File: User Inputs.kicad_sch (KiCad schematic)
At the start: 10 parts, among them SW3 RotaryEncoder_Switch

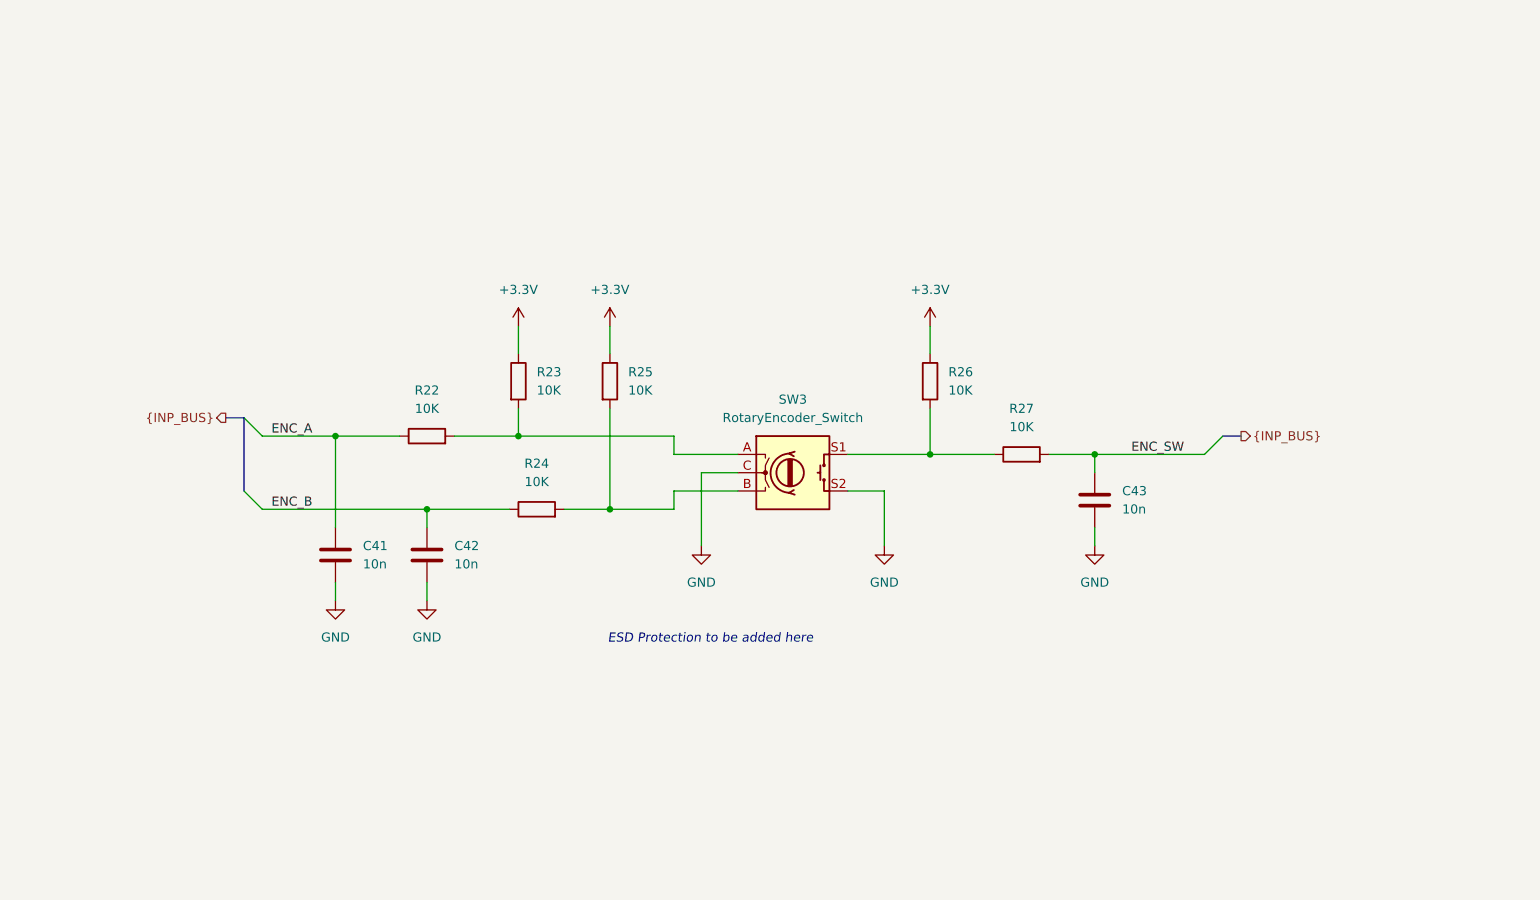
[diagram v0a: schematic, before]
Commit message: Major Changes
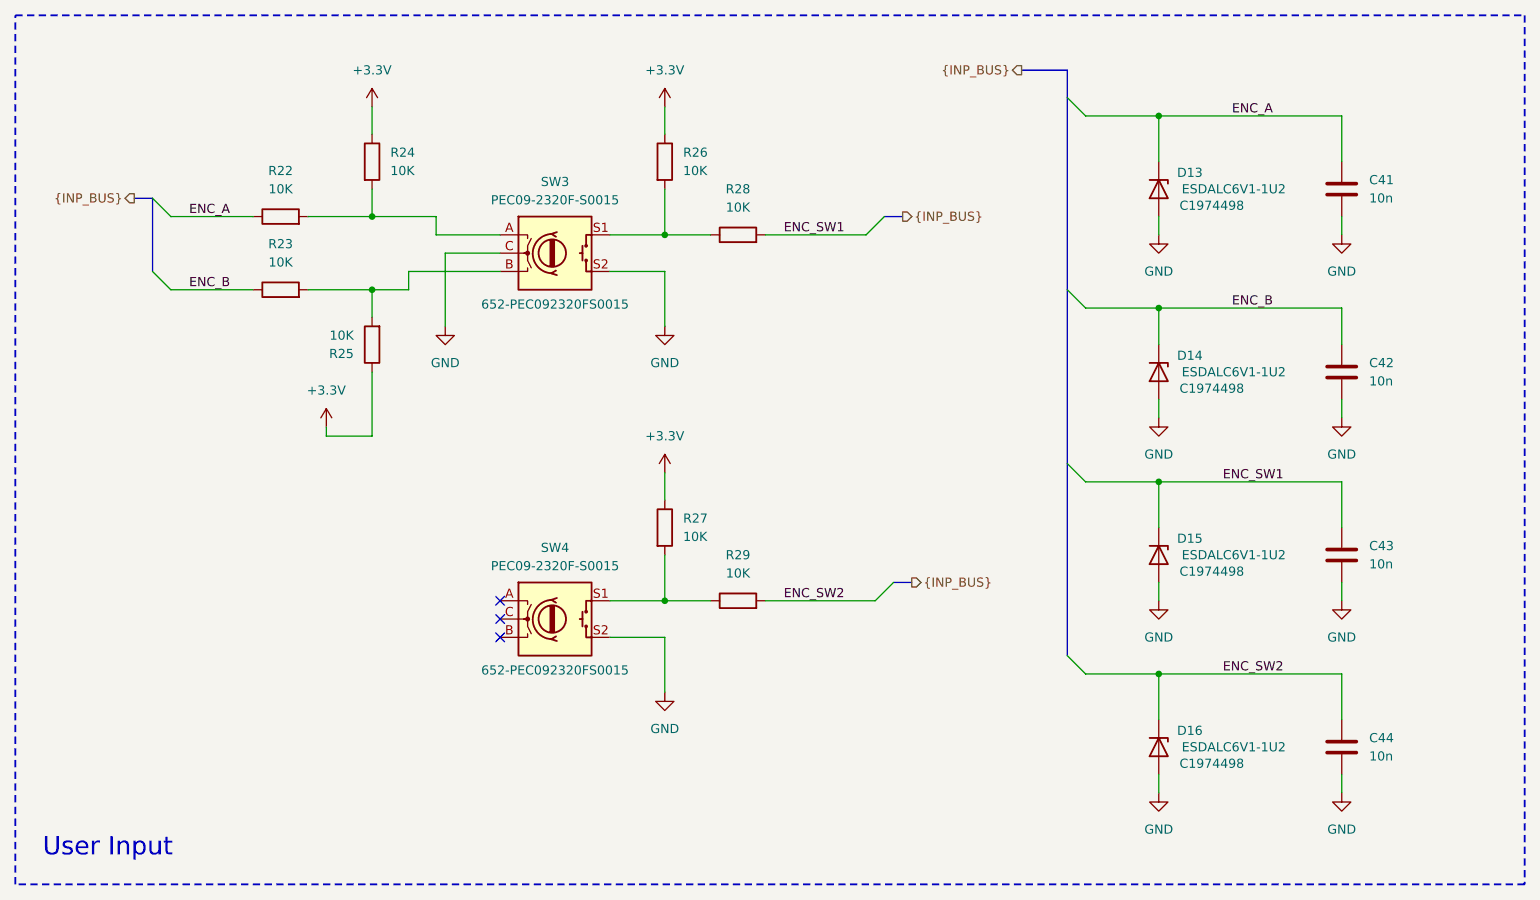
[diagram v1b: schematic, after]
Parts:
- added C44: 10n, Capacitor_SMD:C_0402_1005Metric, symbol Device:C
- added D13, D14, D15, D16: ESDALC6V1-1U2, precision_clock:ST ESDALC6V1-1U2, symbol Diode:ESD5Zxx
- added R27, R29: 10K, Resistor_SMD:R_0402_1005Metric, symbol Device:R
- added SW4: PEC09-2320F-S0015, Rotary_Encoder:RotaryEncoder_Bourns_Horizontal_PEC09-2xxxF-Sxxxx, symbol Device:RotaryEncoder_Switch
- SW3: value RotaryEncoder_Switch -> PEC09-2320F-S0015; footprint (none) -> Rotary_Encoder:RotaryEncoder_Bourns_Horizontal_PEC09-2xxxF-Sxxxx; Mouser (none) -> 652-PEC092320FS0015
- renumbered R24 to R23, R23 to R24, R27 to R28
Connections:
- net +3.3V: now also R27.1
- net ENC_A: now also D13.1 (K)
- net ENC_B: now also D14.1 (K)
- net GND: now also C44.2, D13.2 (A), D14.2 (A), D15.2 (A), D16.2 (A), SW4.S2
- net ENC_SW renamed ENC_SW1
- net ENC_SW1: now also D15.1 (K)
- new net: R27.2, R29.1, SW4.S1
- new net ENC_SW2: C44.1, D16.1 (K), R29.2
- no-connect marks 0 -> 3
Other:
- note added: "User Input"
- note removed: "ESD Protection to be added here"
- moved on the sheet: C41, C42, C43, R22, R23, R24, R25, R26, R28
